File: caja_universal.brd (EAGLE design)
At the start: 100 x 80 mm, 36 parts, among them IC3 TL084P, IC4 TL084P

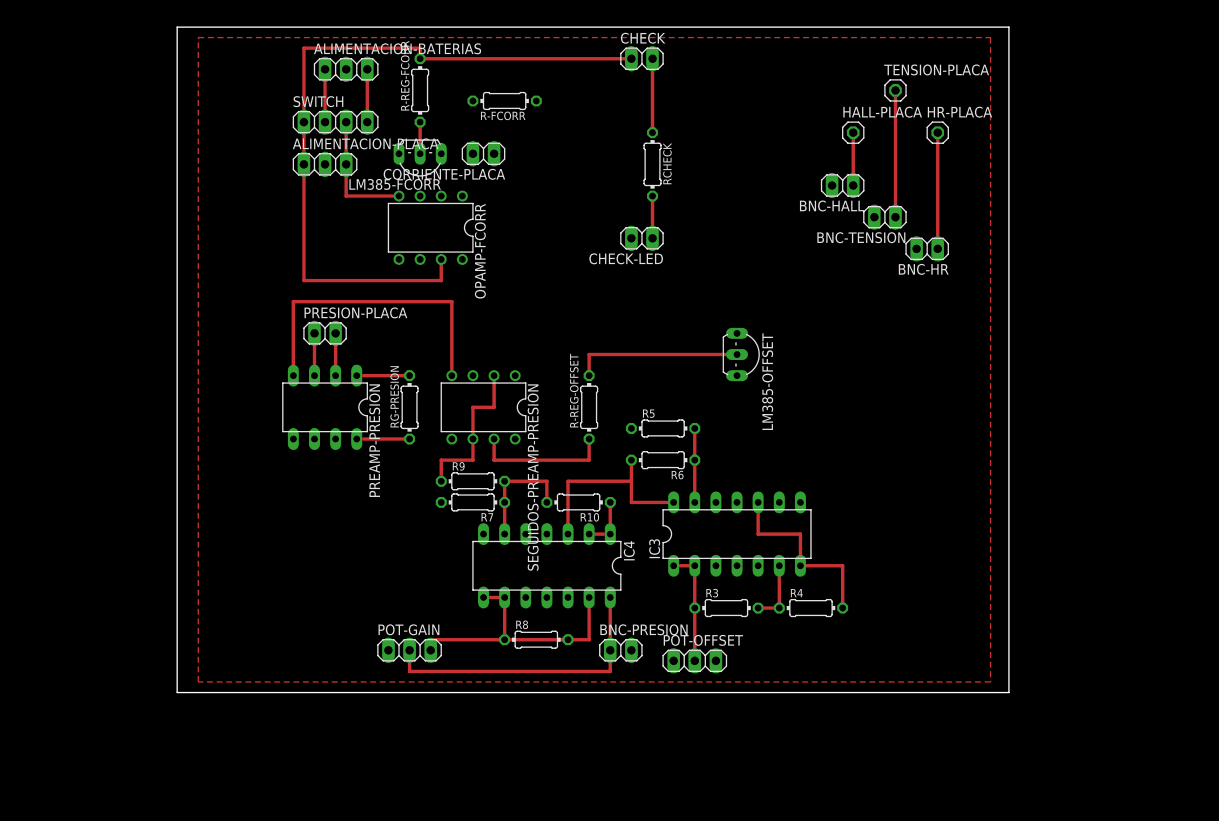
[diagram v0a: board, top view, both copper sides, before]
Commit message: Terminada primera version de la placa
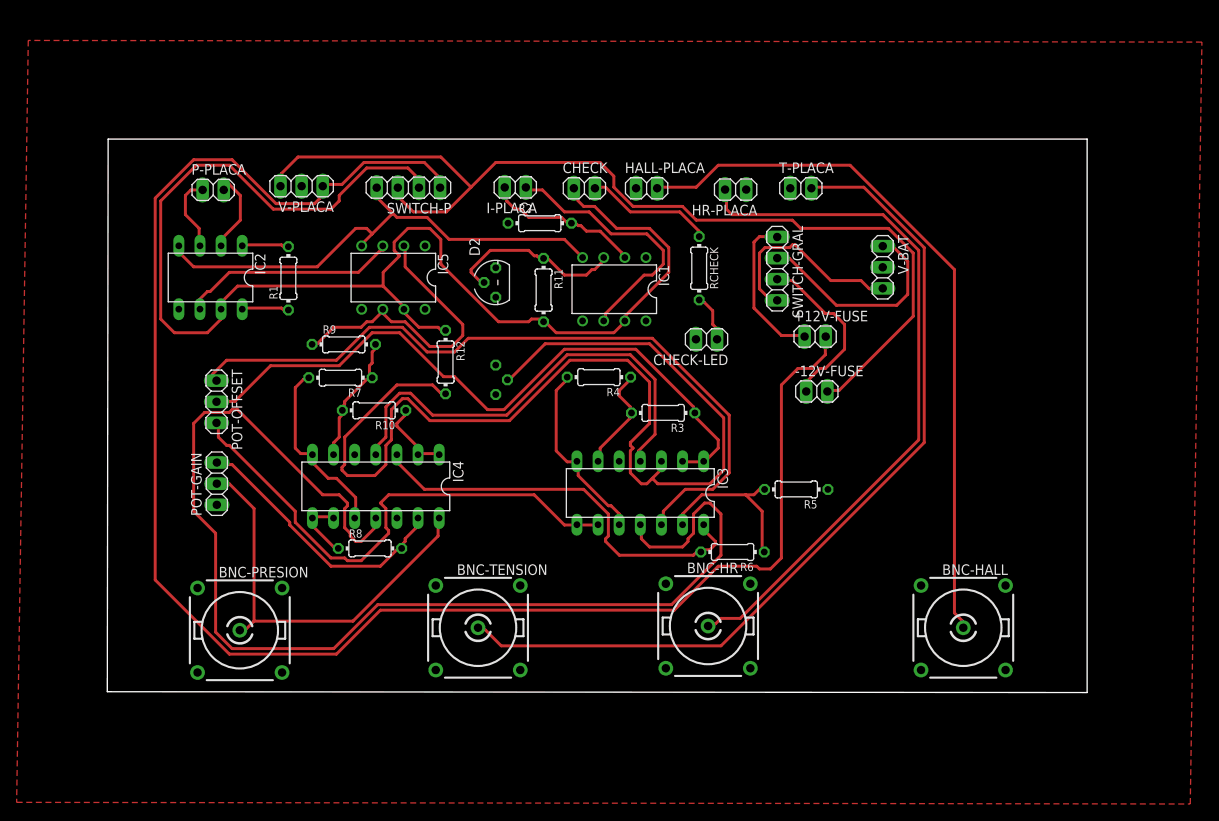
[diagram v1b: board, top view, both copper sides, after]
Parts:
- removed ALIMENTACION-BATERIAS, ALIMENTACION-PLACA: (no value), pinhead:1X03
- removed CORRIENTE-PLACA, PRESION-PLACA: (no value), pinhead:1X02
- removed LM385-FCORR, LM385-OFFSET: 2SC945, transistor:TO92-ECB
- removed OPAMP-FCORR, SEGUIDOS-PREAMP-PRESION: LM318N, linear:DIL08
- removed PREAMP-PRESION: AD620N, analog-devices:DIL08
- removed R-FCORR, RG-PRESION: 820, resistor:0204/7
- removed R-REG-FCORR: 10k, resistor:0204/7
- removed R-REG-OFFSET: 680k, resistor:0204/7
- removed SWITCH: (no value), pinhead:1X04
- removed TENSION-PLACA: (no value), pinhead:1X01
- added +12V-FUSE, -12V-FUSE, I-PLACA, P-PLACA, T-PLACA: (no value), pinhead:1X02
- added D1, D2: LM385, lm385:TO-92
- added IC1, IC5: NE5534AN, linear:DIL08
- added IC2: AD620N, analog-devices:DIL08
- added R1, R2: 820, resistor:0204/7
- added R11: 10k, resistor:0204/7
- added R12: 680k, resistor:0204/7
- added SWITCH-GRAL, SWITCH-P: (no value), pinhead:1X04
- added V-BAT, V-PLACA: (no value), pinhead:1X03
- BNC-HALL, BNC-HR, BNC-PRESION, BNC-TENSION: value (none) -> A1944-50; device pinhead:1X02 -> con-coax:A1944
- HALL-PLACA, HR-PLACA: device pinhead:1X01 -> pinhead:1X02
- moved BNC-TENSION 69.5 mm to (36.2, 7.79), turned to 0 degrees
- moved POT-OFFSET 65.4 mm to (4.73, 35.0), turned to 270 degrees
- moved BNC-HALL 55.1 mm to (94.5, 7.79), turned to 0 degrees
- moved BNC-HR 52.4 mm to (63.8, 8.00), turned to 0 degrees
- moved BNC-PRESION 45.9 mm to (7.53, 7.49)
- moved R4 37.7 mm to (50.7, 37.9), turned to 180 degrees
- moved POT-GAIN 30.6 mm to (4.77, 25.1), turned to 90 degrees
- moved R10 27.0 mm to (23.7, 33.9)
- moved HALL-PLACA 25.7 mm to (56.4, 60.6)
- moved HR-PLACA 25.2 mm to (67.1, 60.5), turned to 180 degrees
- moved R3 24.7 mm to (58.4, 33.6), turned to 180 degrees
- moved R8 22.8 mm to (23.2, 17.3)
- moved IC4 22.7 mm to (23.9, 24.8)
- moved R9 22.6 mm to (20.0, 41.9)
- moved R7 21.9 mm to (19.6, 37.9)
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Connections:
- net PRESION renamed POUT
- removed net 0VBAT: ALIMENTACION-BATERIAS.2
- removed net PRESION-PREAMP: PREAMP-PRESION.6, SEGUIDOS-PREAMP-PRESION.3
- new net +12V-PRESION: CHECK.1, IC1.7, IC2.7, IC5.7, R11.2, R12.1, SWITCH-P.2
- new net +12VFUSE: +12V-FUSE.1, SWITCH-GRAL.1
- new net -12V-PRESION: IC1.4, IC2.4, IC5.4, SWITCH-P.4
- new net -12VFUSE: -12V-FUSE.1, SWITCH-GRAL.3
- new net P-PREAMP: IC2.6, IC5.3
- net +12V: now also +12V-FUSE.2, SWITCH-P.1, V-PLACA.1; no longer ALIMENTACION-PLACA.1, CHECK.1, OPAMP-FCORR.7, PREAMP-PRESION.7, R-REG-FCORR.2, R-REG-OFFSET.1, SEGUIDOS-PREAMP-PRESION.7, SWITCH.1
- net +12VBAT: now also SWITCH-GRAL.2, V-BAT.1; no longer ALIMENTACION-BATERIAS.1, SWITCH.2
- net +I: now also I-PLACA.1, IC1.6; no longer CORRIENTE-PLACA.1, OPAMP-FCORR.6
- net -12V: now also -12V-FUSE.2, SWITCH-P.3, V-PLACA.3; no longer ALIMENTACION-PLACA.3, OPAMP-FCORR.4, PREAMP-PRESION.4, SEGUIDOS-PREAMP-PRESION.4, SWITCH.3
- net -12VBAT: now also SWITCH-GRAL.4, V-BAT.3; no longer ALIMENTACION-BATERIAS.3, SWITCH.4
- net -I: now also I-PLACA.2, IC1.2, R2.2; no longer CORRIENTE-PLACA.2, OPAMP-FCORR.2, R-FCORR.2
- net 0V: now also BNC-HALL.3, BNC-HALL.4, BNC-HALL.5, BNC-HR.3, BNC-HR.4, BNC-HR.5, BNC-PRESION.3, BNC-PRESION.4, BNC-PRESION.5, BNC-TENSION.3, BNC-TENSION.4, BNC-TENSION.5, D1.-, D1.FB, D2.-, D2.FB, IC2.5, R2.1, V-BAT.2, V-PLACA.2; no longer ALIMENTACION-PLACA.2, LM385-FCORR.B, LM385-FCORR.E, LM385-OFFSET.B, LM385-OFFSET.E, PREAMP-PRESION.5, R-FCORR.1
- net HALL: now also HALL-PLACA.2; no longer HALL-PLACA.1
- net HR: now also HR-PLACA.2; no longer HR-PLACA.1
- net N$13: now also IC5.2, IC5.6; no longer SEGUIDOS-PREAMP-PRESION.2, SEGUIDOS-PREAMP-PRESION.6
- net N$3: now also D2.+, IC1.3, R11.1; no longer LM385-FCORR.C, OPAMP-FCORR.3, R-REG-FCORR.1
- net N$4: now also IC2.1, R1.2; no longer PREAMP-PRESION.1, RG-PRESION.2
- net N$5: now also IC2.8, R1.1; no longer PREAMP-PRESION.8, RG-PRESION.1
- net N$7: now also D1.+, R12.2; no longer LM385-OFFSET.C, R-REG-OFFSET.2
- net P+: now also IC2.3, P-PLACA.1; no longer PREAMP-PRESION.3, PRESION-PLACA.1
- net P-: now also IC2.2, P-PLACA.2; no longer PREAMP-PRESION.2, PRESION-PLACA.2
- net TENSION: now also T-PLACA.2; no longer TENSION-PLACA.1
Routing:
- net +12V-PRESION: track 0.00 -> 163.9 mm
- net V-: track 0.00 -> 146.7 mm
- net N$7: track 20.3 -> 134.4 mm
- net +12V: track 104.1 -> 203.0 mm
- net OFFSET: track 0.00 -> 89.6 mm
- net TENSION: track 15.2 -> 104.8 mm
- net HALL: track 6.35 -> 85.6 mm
- net HR: track 14.0 -> 85.0 mm
- net -12V: track 52.1 -> 119.9 mm
- net 1.25V: track 14.0 -> 81.7 mm
- net -1.25V: track 0.00 -> 62.8 mm
- net -12V-PRESION: track 0.00 -> 61.4 mm
- net V+: track 0.00 -> 55.4 mm
- net +I: track 0.00 -> 31.9 mm
- net P-PREAMP: track 0.00 -> 26.8 mm
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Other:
- board size 100 x 80 mm -> 117.8 x 66.5 mm
